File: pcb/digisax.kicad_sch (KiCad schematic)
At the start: 62 parts, among them J1 Conn_01x04_Pin, J2 Conn_01x04_Pin, J3 Conn_01x05_Pin, J4 Conn_01x05_Pin, J5 Conn_01x04_Pin, J6 Conn_01x04_Pin, J7 Conn_01x03_Pin, J8 Conn_01x03_Pin, J9 Barrel_Jack, SW1 RotaryEncoder_Switch, U1 ER_OLEDM0.91_1x-I2C, U2 MPXV7007, U3 MCP3221, U4 TLV320DAC3100_breakout, U5 ESP32-S3

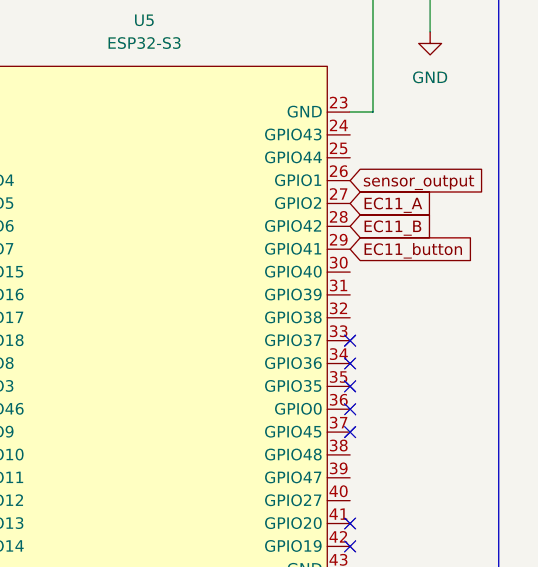
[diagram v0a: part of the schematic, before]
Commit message: had a go at routing
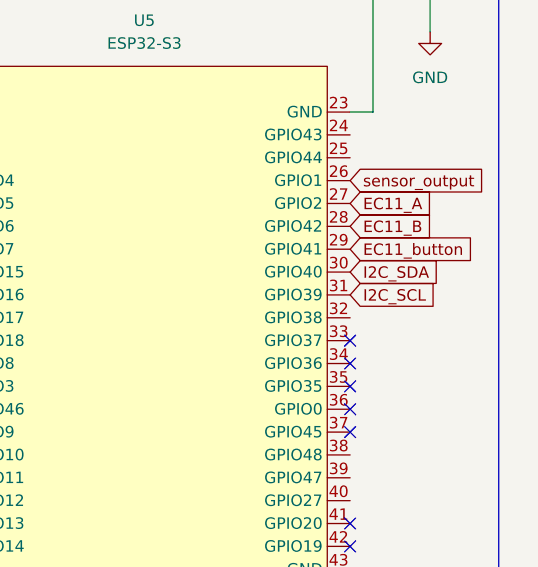
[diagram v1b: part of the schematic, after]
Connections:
- net I2C_SCL: now also U5.31 (GPIO39)
- net I2C_SDA: now also U5.30 (GPIO40)
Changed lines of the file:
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@@
+		)
+	)
+	(global_label "I2C_SDA"
+		(shape input)
+		(at 370.84 81.28 0)
+		(fields_autoplaced yes)
+		(effects
+			(font
+				(size 1.27 1.27)
+			)
+			(justify left)
+		)
+		(property "Intersheetrefs" "${INTERSHEET_REFS}"
+			(at 381.4452 81.28 0)
+			(hide yes)
+			(show_name no)
+			(do_not_autoplace no)
+			(effects
+				(font
+					(size 1.27 1.27)
+				)
+				(justify left)
+			)
 		)
 	)
@@
 			)
 		)
+	)
+	(global_label "I2C_SCL"
+		(shape input)
+		(at 370.84 83.82 0)
+		(fields_autoplaced yes)
+		(effects
+			(font
+				(size 1.27 1.27)
+			)
+			(justify left)
+		)
+		(property "Intersheetrefs" "${INTERSHEET_REFS}"
+			(at 381.3847 83.82 0)
+			(hide yes)
+			(show_name no)
+			(do_not_autoplace no)
+			(effects
+				(font
+					(size 1.27 1.27)
+				)
+				(justify left)
+			)
+		)
